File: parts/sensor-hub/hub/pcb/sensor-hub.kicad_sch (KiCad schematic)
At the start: 10 parts, among them J1 MPT1584 buck, J2 PWR IN, SW2 SW_SPDT, U1 ESP32 Wemos D1 Mini

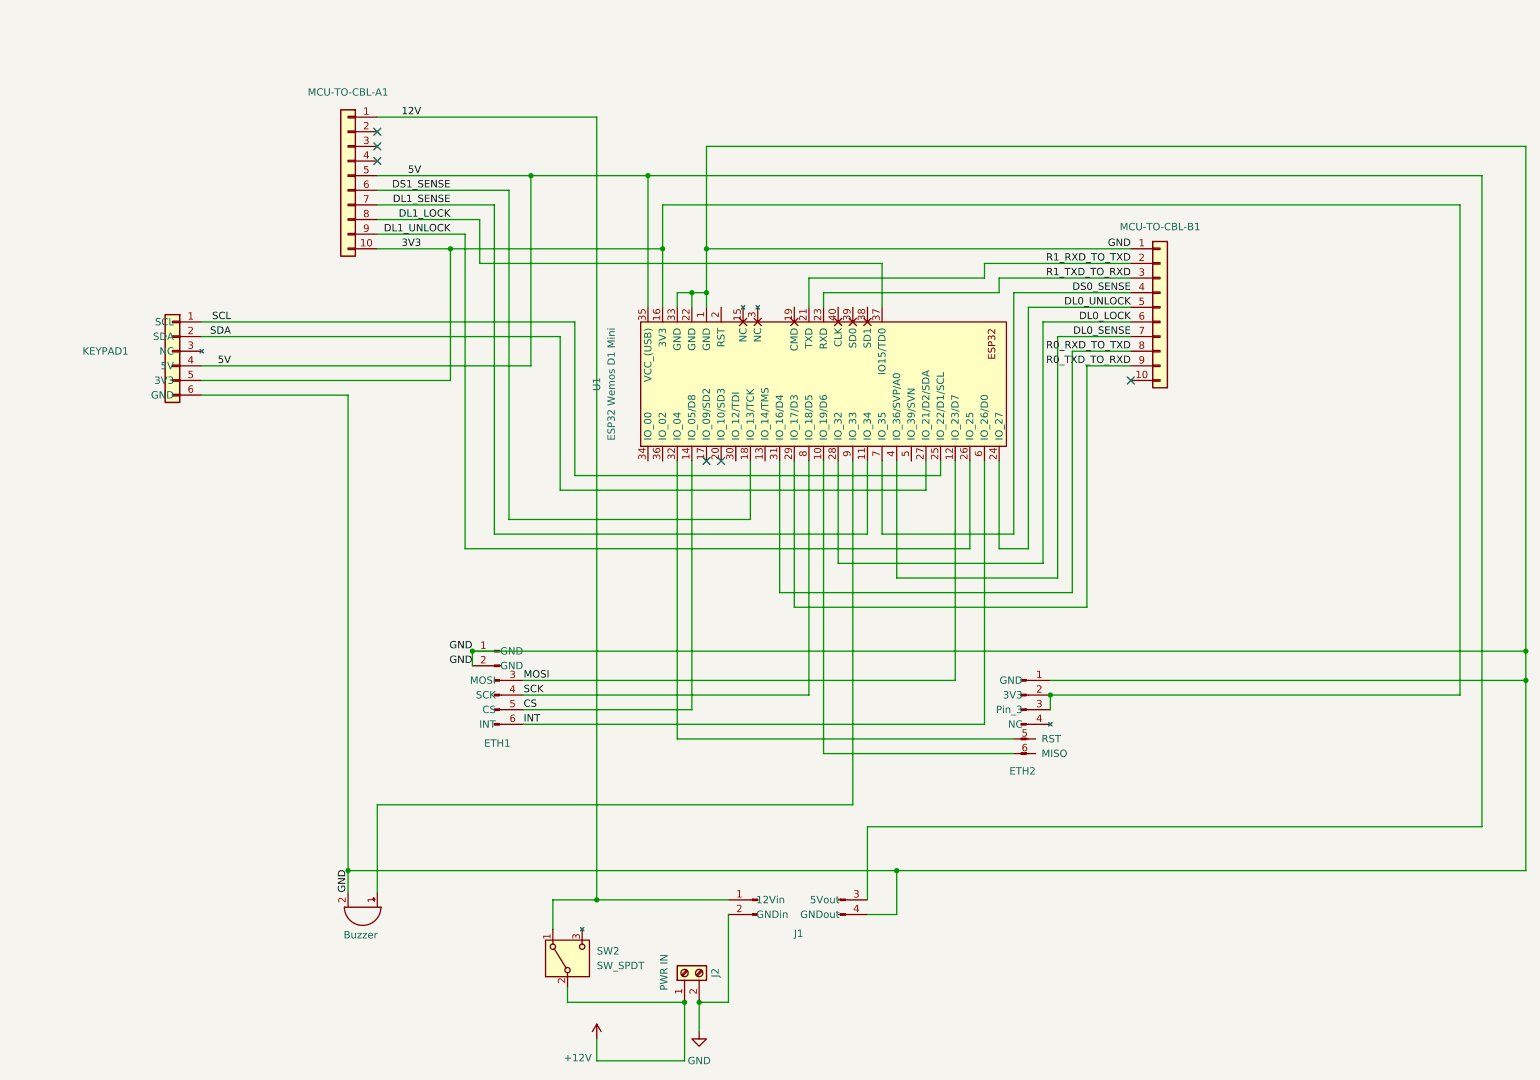
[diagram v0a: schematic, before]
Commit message: hub 7.0
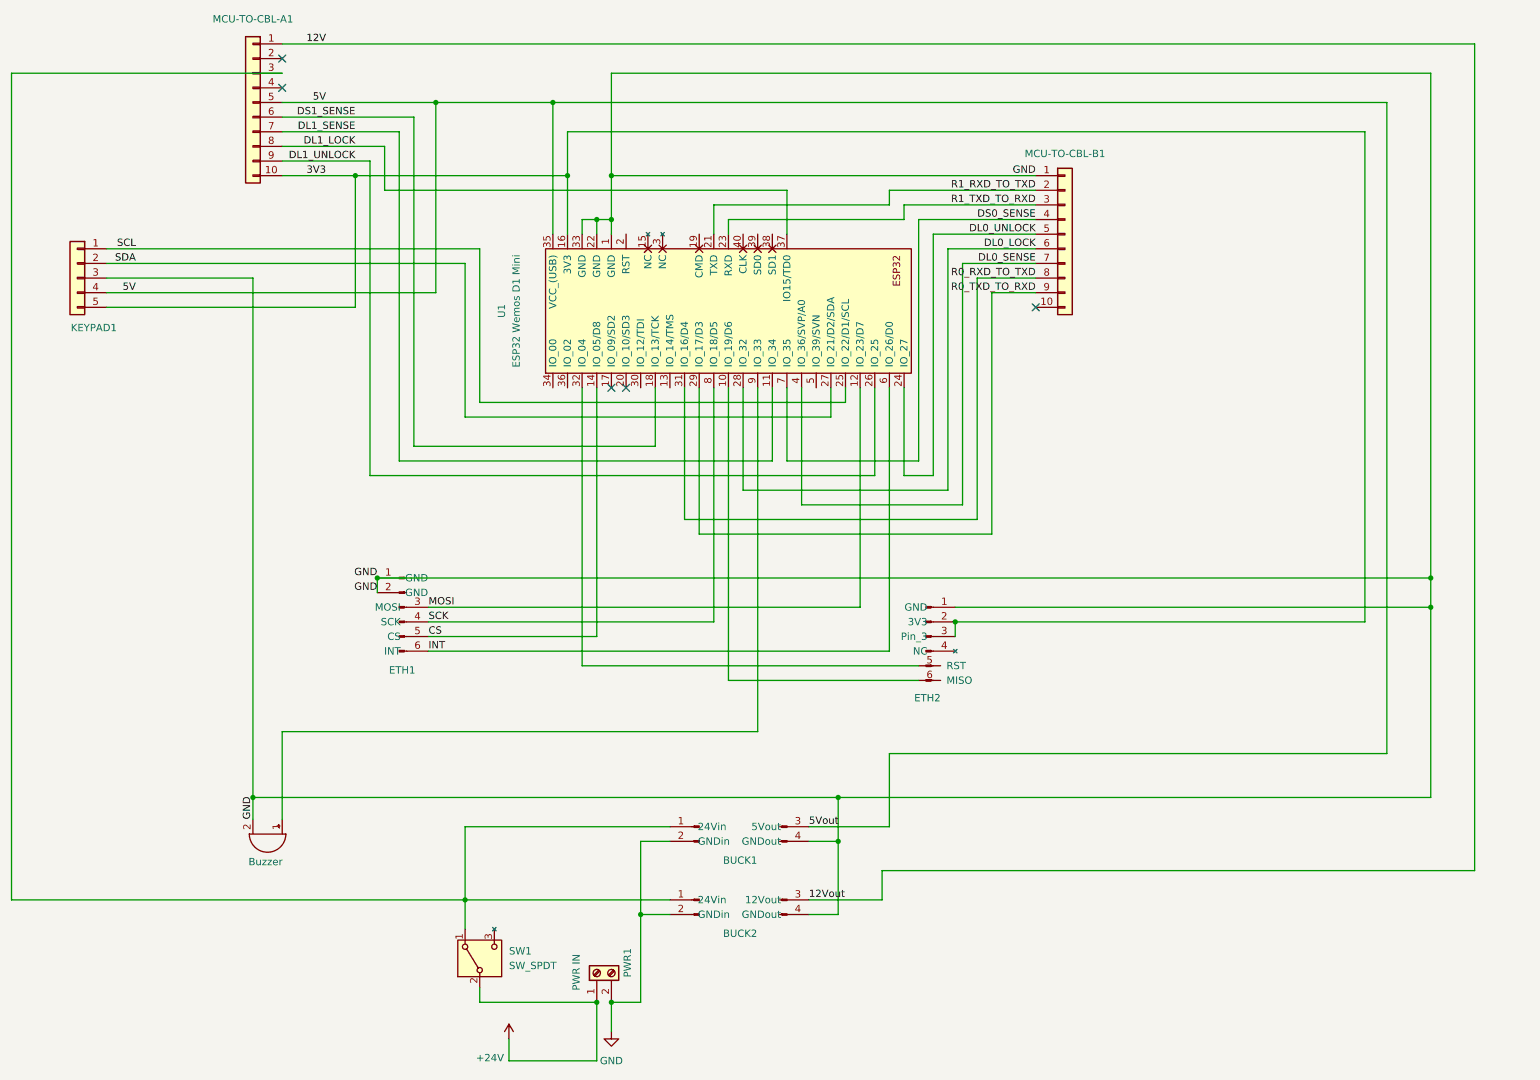
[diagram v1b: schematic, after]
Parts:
- added BUCK2: MPT1584 buck, local_project:SRT_MPT1584EN_Module, symbol Connector:Conn_01x04_Pin
- BUCK1: renamed from J1; footprint sensor hub.04:SRT_MPT1584EN_Module -> local_project:SRT_MPT1584EN_Module
- KEYPAD1: value Conn_01x06 -> Conn_01x05; footprint Connector_PinHeader_2.54mm:PinHeader_1x06_P2.54mm_Horizontal -> Connector_PinHeader_2.54mm:PinHeader_1x05_P2.54mm_Horizontal; symbol Connector_Generic:Conn_01x06 -> Connector_Generic:Conn_01x05
- U1: footprint sensor hub.04:esp32-wemos-d1-mini -> local_project:esp32-wemos-d1-mini
- renumbered J2 to PWR1, SW2 to SW1
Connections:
- net 12V: now also BUCK2.3 (12Vout); no longer BUCK1.1 (12Vin), SW1.1 (A)
- net GND: now also KEYPAD1.3 (Pin_3), BUCK2.2 (GNDin), BUCK2.4 (GNDout); no longer KEYPAD1.6 (GND)
- net at MCU-TO-CBL-A1.3 (Pin_3): now also BUCK1.1 (24Vin), SW1.1 (A), BUCK2.1 (24Vin)
- net +12V renamed +24V
- no-connect marks 6 -> 5
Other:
- moved on the sheet: BUCK1, ETH1, ETH2, MCU-TO-CBL-A1, MCU-TO-CBL-B1, PWR1, SW1, U1
